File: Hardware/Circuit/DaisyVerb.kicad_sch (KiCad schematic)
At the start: 34 parts, among them J1 AUDIO_IN1, J2 AUDIO_OUT1, J3 AUDIO_IN1, J4 AUDIO_OUT2, U1 TL074, U2 TL074

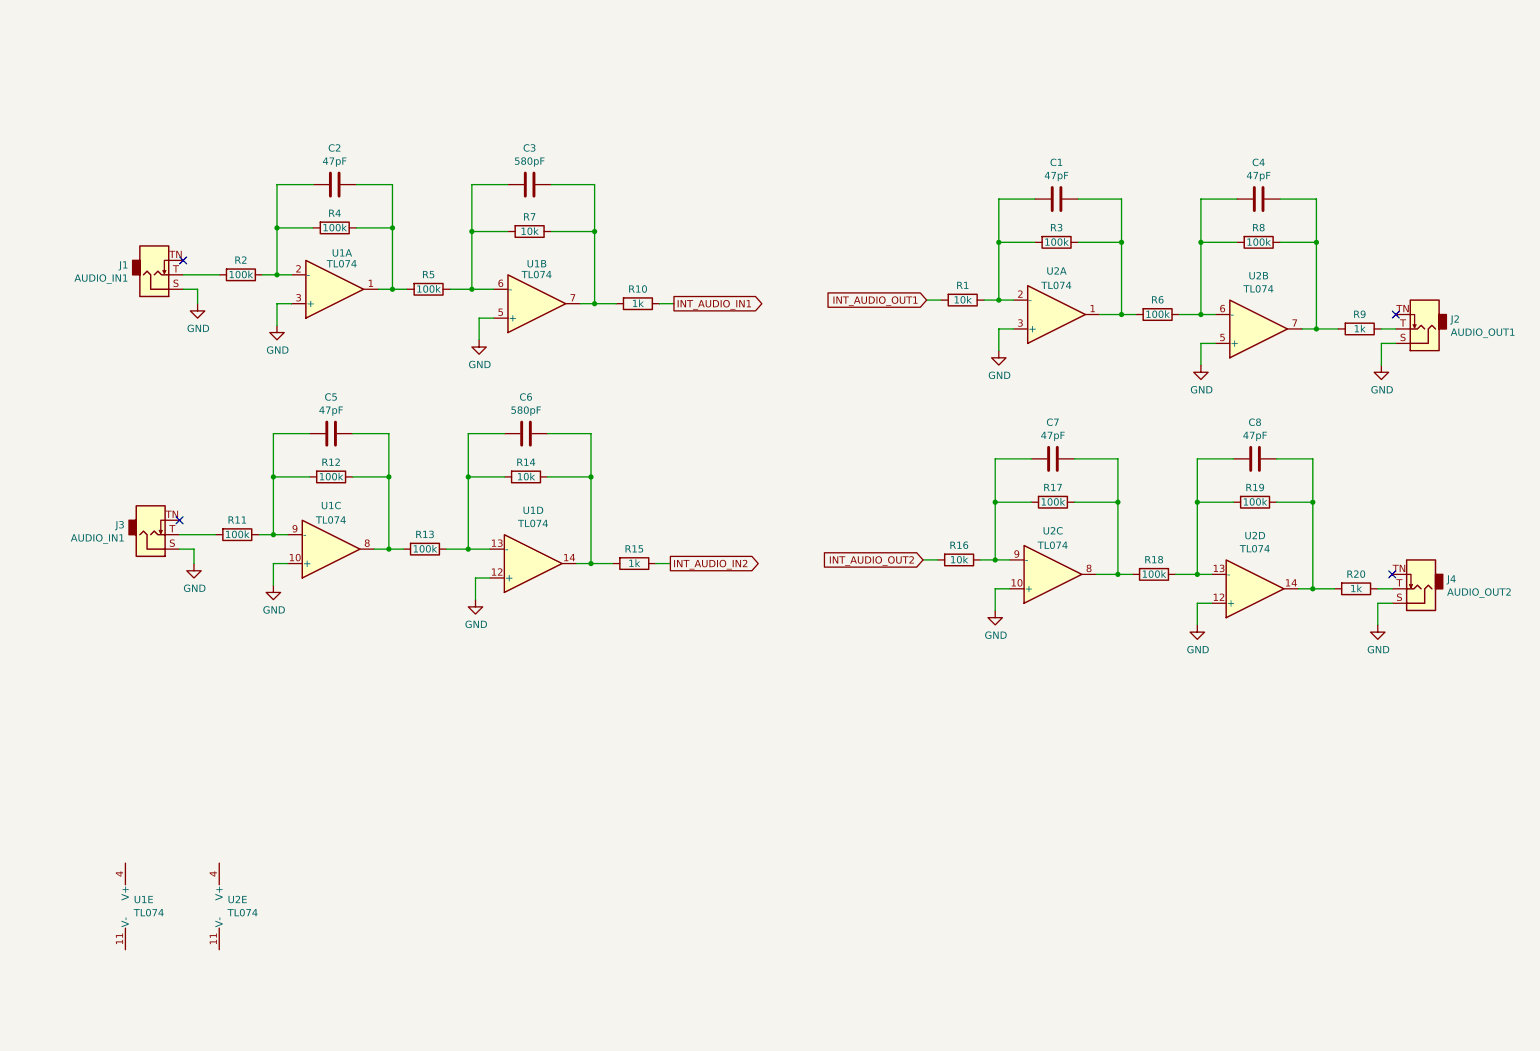
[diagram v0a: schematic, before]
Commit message: Completed schematics
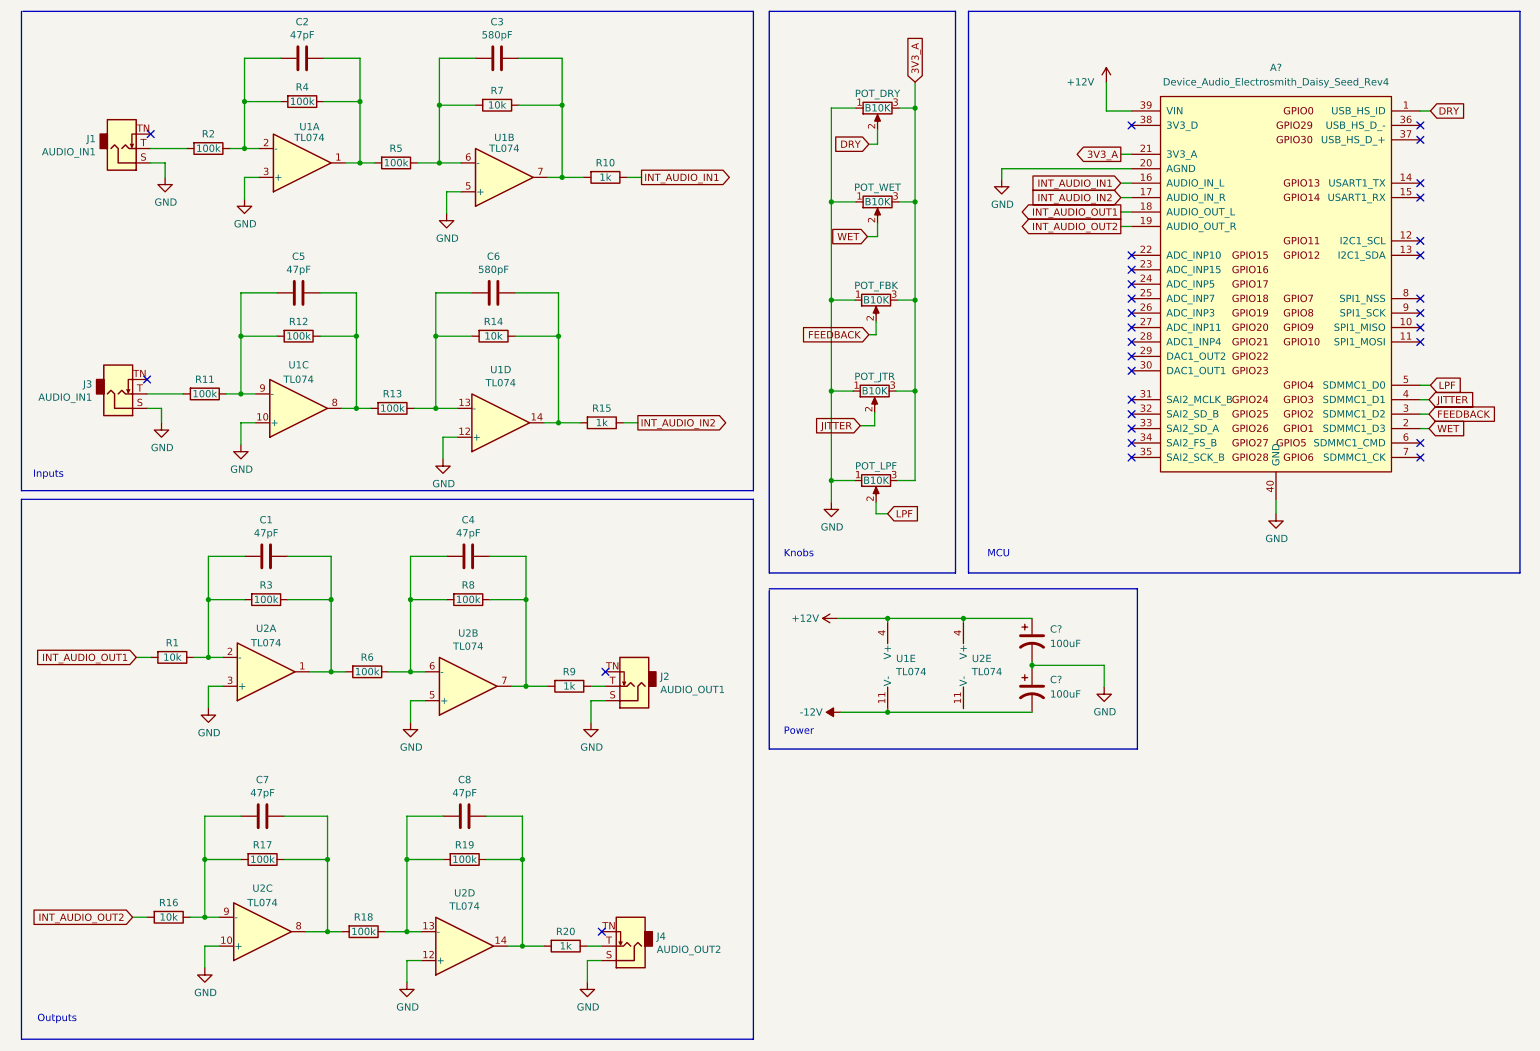
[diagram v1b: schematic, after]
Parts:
- added A?: Device_Audio_Electrosmith_Daisy_Seed_Rev4, daisy-seed:Device_Audio_Electrosmith_Daisy_Seed, symbol Device_Audio_Electrosmith_Daisy_Seed:Device_Audio_Electrosmith_Daisy_Seed_Rev4
- added C? (x2): 100uF, symbol Device:C_Polarized_US
- added POT_DRY, POT_FBK, POT_JTR, POT_LPF, POT_WET: B10K, symbol Device:R_Potentiometer
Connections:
- net GND: now also A?.20 (AGND), A?.40 (GND), C?.1, C?.2, POT_DRY.1, POT_FBK.1, POT_JTR.1, POT_LPF.1, POT_WET.1
- net INT_AUDIO_IN1: now also A?.16 (AUDIO_IN_L)
- net INT_AUDIO_IN2: now also A?.17 (AUDIO_IN_R)
- net INT_AUDIO_OUT1: now also A?.18 (AUDIO_OUT_L)
- net INT_AUDIO_OUT2: now also A?.19 (AUDIO_OUT_R)
- net -12V: now reaches U1.11 (V-)
- net -12V: now also C?.2
- net +12V: now reaches U1.4 (V+)
- net +12V: now also U2.4 (V+), A?.39 (VIN), C?.1
- new net 3V3_A: A?.21 (3V3_A), POT_DRY.3, POT_FBK.3, POT_JTR.3, POT_LPF.3, POT_WET.3
- new net DRY: A?.1 (USB_HS_ID), POT_DRY.2
- new net FEEDBACK: A?.3 (SDMMC1_D2), POT_FBK.2
- new net JITTER: A?.4 (SDMMC1_D1), POT_JTR.2
- new net LPF: A?.5 (SDMMC1_D0), POT_LPF.2
- new net WET: A?.2 (SDMMC1_D3), POT_WET.2
- no-connect marks 4 -> 31
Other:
- note added: "Inputs"
- note added: "Knobs"
- note added: "MCU"
- note added: "Outputs"
- note added: "Power"
- moved on the sheet: C1, C2, C3, C4, C5, C6, C7, C8, J1, J2, J3, J4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
